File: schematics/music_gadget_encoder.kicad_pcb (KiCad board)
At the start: 2 copper layers, 96.5 x 49.9 mm, 249 parts, among them IC1 TLC5926IPWPR, J6 Conn_01x02_Male, Q1 DMG9933USD-13, Q2 DMG9933USD-13, Q3 DMG9933USD-13, Q4 DMG9933USD-13, Q5 DMG9933USD-13, SW1 SW_Push, SW2 SW_Push, SW3 SW_Push, SW4 SW_Push, SW5 SW_Push, SW6 SW_Push, SW7 SW_Push, U1 STM32G070CBTx, U2 PEC12R-4225F-S0024, U3 PEC12R-4225F-S0024, U4 PEC12R-4225F-S0024, U5 PEC12R-4225F-S0024, Y1 Crystal_GND24

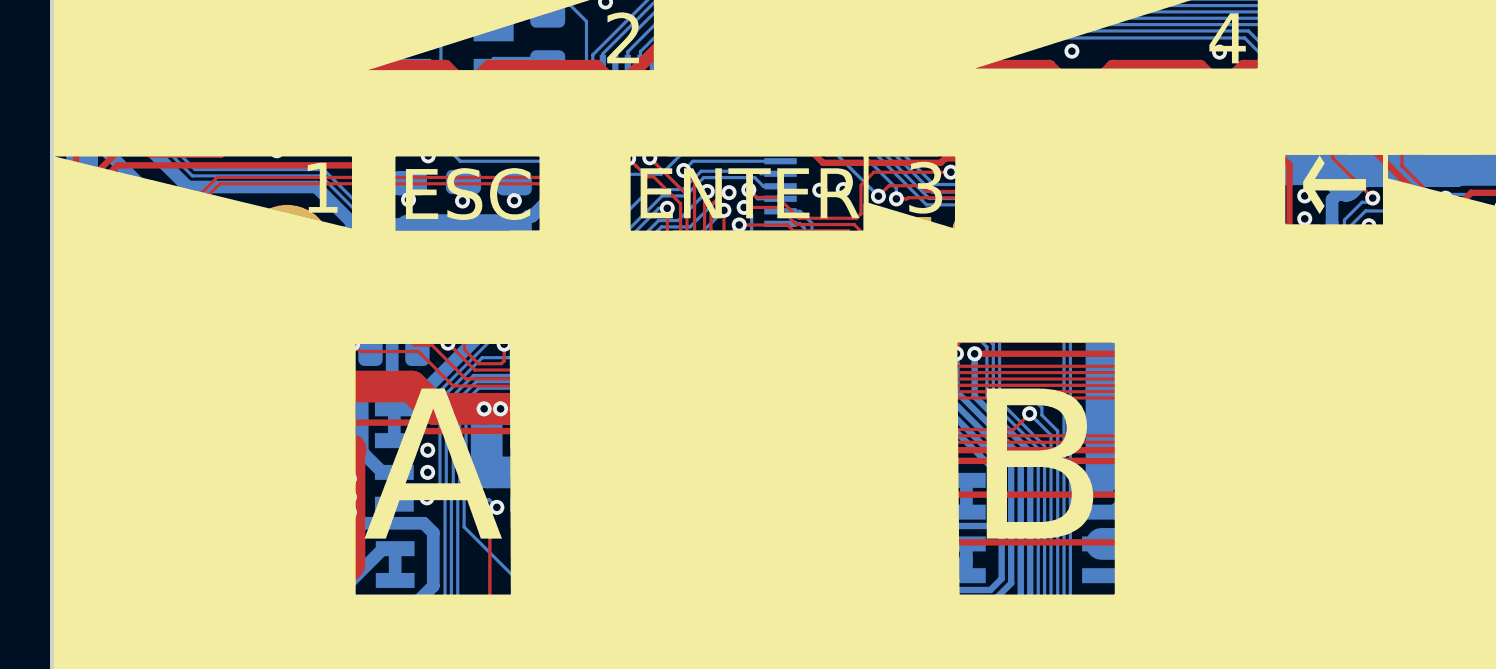
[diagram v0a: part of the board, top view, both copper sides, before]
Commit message: update pcb
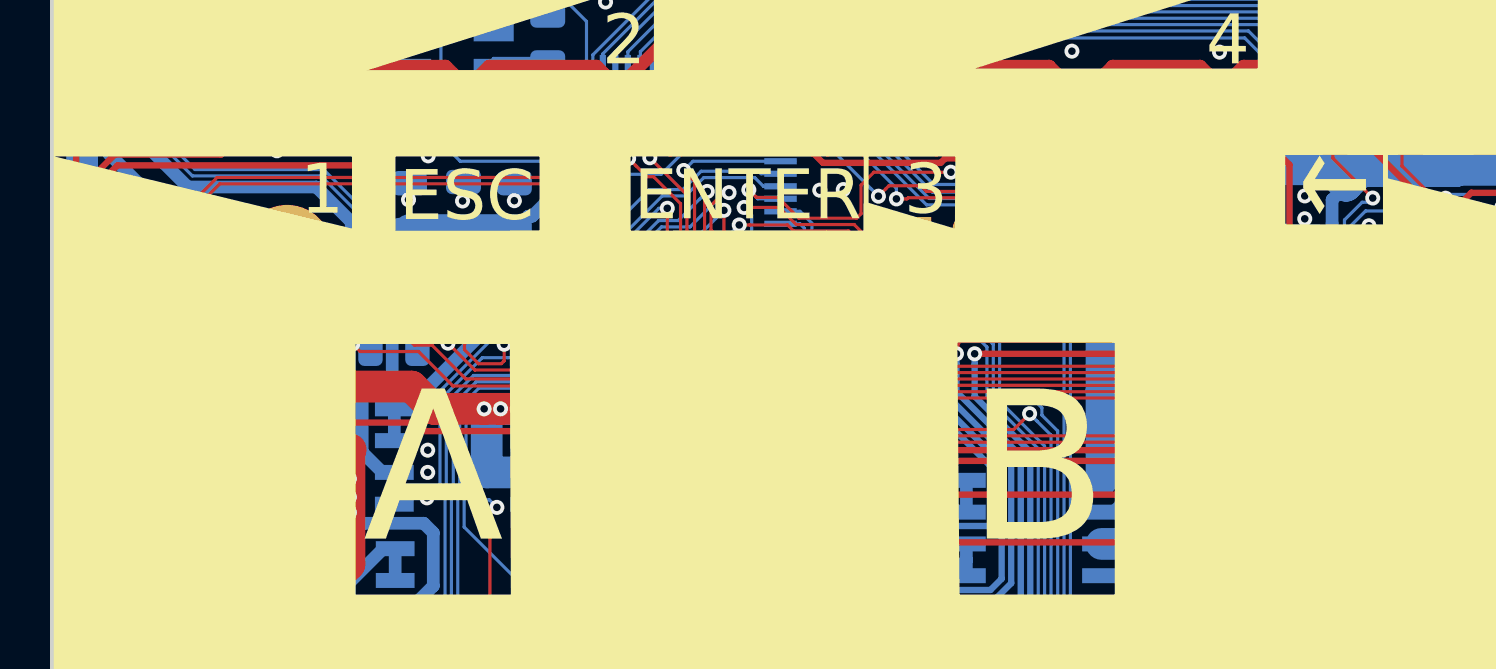
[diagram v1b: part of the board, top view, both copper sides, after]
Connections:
- J_LEFT1 pad 3: /USART4_RX -> /USART4_TX
- J_LEFT1 pad 4: /USART4_TX -> /USART4_RX
- J_TOP1 pad 3: /USART3_RX -> /USART3_TX
- J_TOP1 pad 4: /USART3_TX -> /USART3_RX
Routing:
- net /USART3_TX: track 20.1 -> 25.4 mm
- net /USART4_TX: track 32.3 -> 35.5 mm
- net /USART3_RX: track 16.1 -> 19.0 mm
- net /USART4_RX: track 35.4 -> 33.3 mm
- net VCC: track 500.7 -> 499.0 mm
- net GND: vias 246 -> 244
